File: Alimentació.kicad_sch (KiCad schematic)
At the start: 26 parts, among them J1 USB_C_Receptacle_PowerOnly_6P, U2 BQ25628ERYKR, U3 TLV61048DBVR, U4 TLV61070ADBV

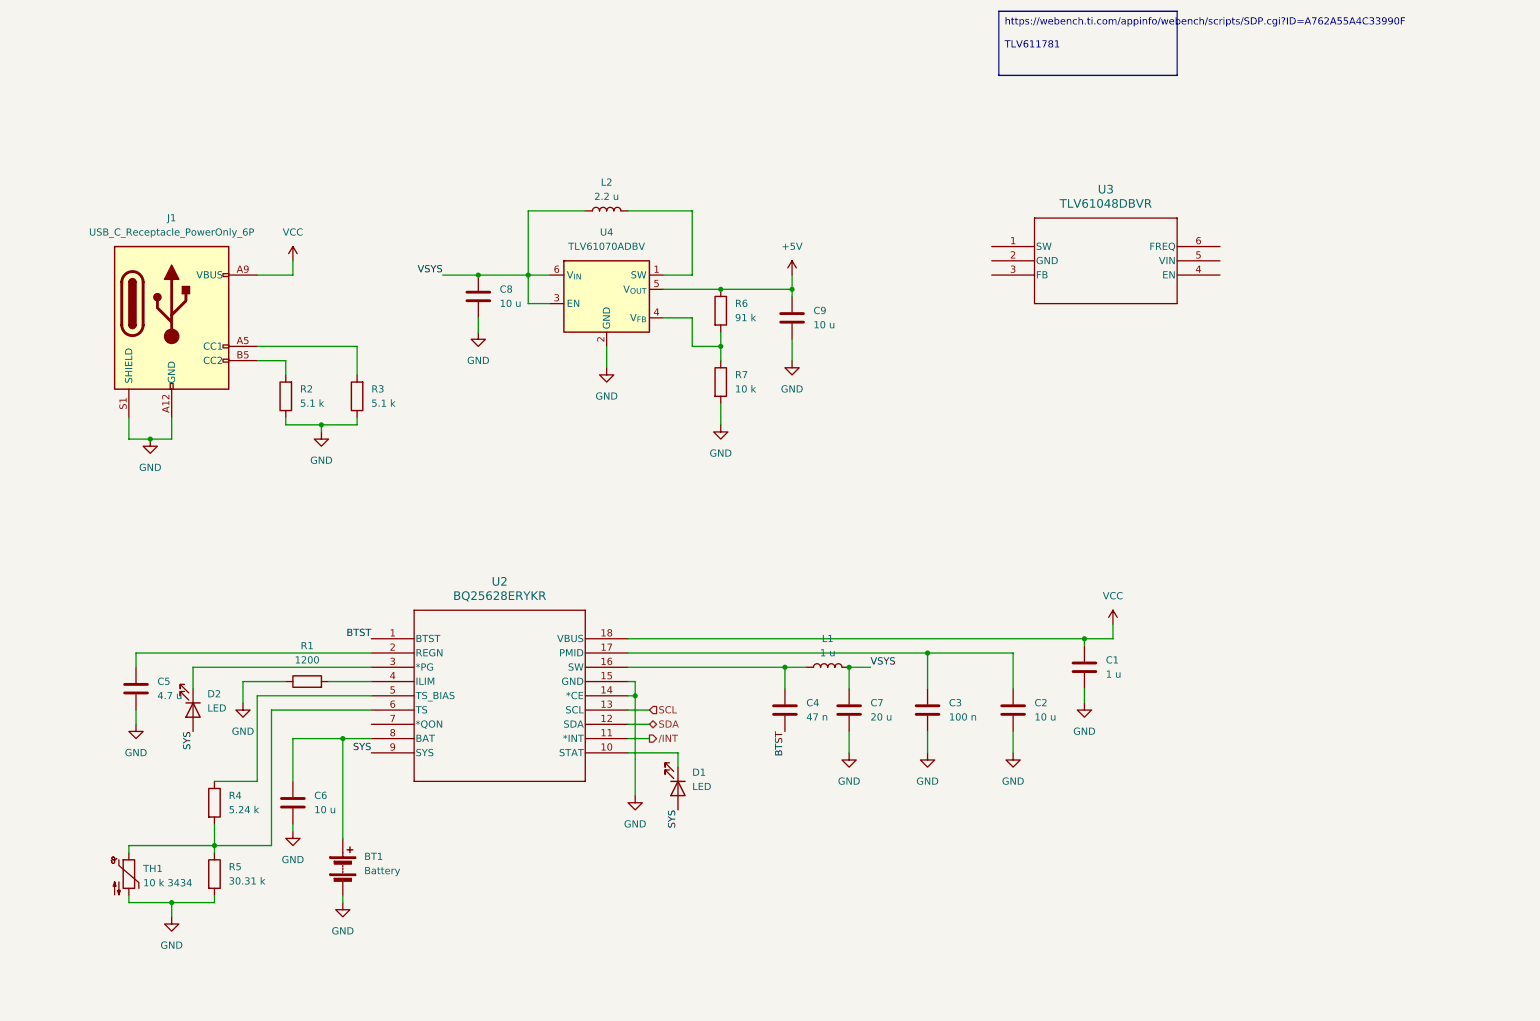
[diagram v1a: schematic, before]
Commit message: actualitzar ultrima versio pcb/esquematic
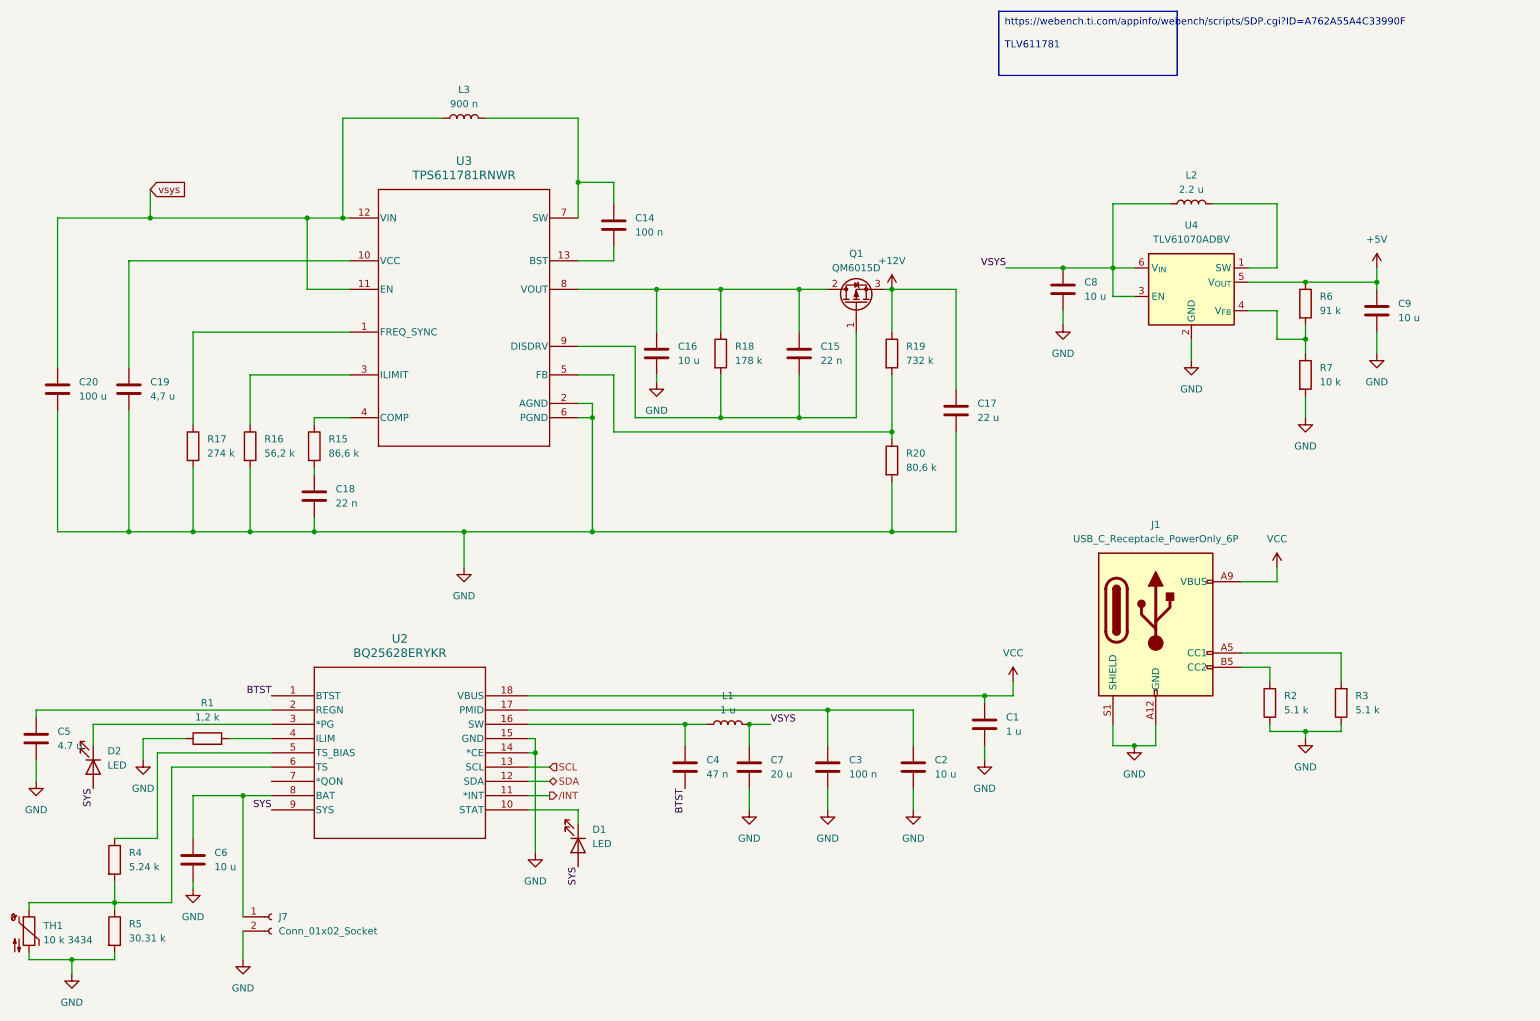
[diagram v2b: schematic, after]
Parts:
- removed BT1: Battery, symbol Device:Battery
- removed U3: TLV61048DBVR, SOT-23-6_DBV_TEX, symbol TLV61048:TLV61048DBVR
- added C14: 100 n, Capacitor_SMD:C_0201_0603Metric, symbol Device:C
- added C15, C18: 22 n, Capacitor_SMD:C_0201_0603Metric, symbol Device:C
- added C16: 10 u, Capacitor_SMD:C_0201_0603Metric, symbol Device:C
- added C17: 22 u, Capacitor_SMD:C_0201_0603Metric, symbol Device:C
- added C19: 4,7 u, Capacitor_SMD:C_0201_0603Metric, symbol Device:C
- added C20: 100 u, Capacitor_SMD:C_0201_0603Metric, symbol Device:C
- added J7: Conn_01x02_Socket, Connector_JST:JST_PH_B2B-PH-K_1x02_P2.00mm_Vertical, symbol Connector:Conn_01x02_Socket
- added L3: 900 n, Inductor_SMD:L_1008_2520Metric_Pad1.43x2.20mm_HandSolder, symbol Device:L
- added Q1: QM6015D, Package_TO_SOT_SMD:TO-252-2, symbol Transistor_FET:QM6015D
- added R15: 86,6 k, Resistor_SMD:R_0201_0603Metric, symbol Device:R
- added R16: 56,2 k, Resistor_SMD:R_0201_0603Metric, symbol Device:R
- added R17: 274 k, Resistor_SMD:R_0201_0603Metric, symbol Device:R
- added R18: 178 k, Resistor_SMD:R_0201_0603Metric, symbol Device:R
- added R19: 732 k, Resistor_SMD:R_0201_0603Metric, symbol Device:R
- added R20: 80,6 k, Mounting_Wuerth:Mounting_Wuerth_WA-SMSE-ExternalM3_H6mm_9771060360, symbol Device:R
- added U3: TPS611781RNWR, RNW0013A, symbol TPS61178:TPS611781RNWR
- C8, C9: footprint (none) -> Capacitor_SMD:C_0201_0603Metric
- D1, D2: footprint (none) -> Diode_SMD:D_0201_0603Metric
- J1: footprint (none) -> USBC_6_DEALON:USB_C_6_DEALON
- L1, L2: footprint (none) -> Inductor_SMD:L_1008_2520Metric_Pad1.43x2.20mm_HandSolder
- R1: value 1200 -> 1,2 k; footprint (none) -> Resistor_SMD:R_0201_0603Metric
- R2, R3, R4, R5, R6, R7, TH1: footprint (none) -> Resistor_SMD:R_0201_0603Metric
- U2: footprint WQFN-HR18__RYK_TEX -> BQ25628E:WQFN-HR18__RYK_TEX
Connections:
- net GND: now also C16.2, C17.2, C18.2, C19.2, C20.2, J7.2 (Pin_2), R16.2, R17.2, R20.2, U3.2 (AGND), U3.6 (PGND)
- net at C6.1, U2.8 (BAT): now also J7.1 (Pin_1)
- new net: C19.1, U3.10 (VCC)
- new net: R17.1, U3.1 (FREQ_SYNC)
- new net: C14.2, U3.13 (BST)
- new net: R16.1, U3.3 (ILIMIT)
- new net: R15.1, U3.4 (COMP)
- new net: R19.2, R20.1, U3.5 (FB)
- new net: C14.1, L3.2, U3.7 (SW)
- new net: C15.1, C16.1, Q1.2 (D), R18.1, U3.8 (VOUT)
- new net: C15.2, Q1.1 (G), R18.2, U3.9 (DISDRV)
- new net: C18.1, R15.2
- new net +12V: C17.1, Q1.3 (S), R19.1
- new net vsys: C20.1, L3.1, U3.11 (EN), U3.12 (VIN)
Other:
- moved on the sheet: C1, C2, C3, C4, C5, C6, C7, C8, C9, D1, D2, J1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
